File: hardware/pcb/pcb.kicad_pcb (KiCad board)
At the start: 2 copper layers, 20 parts, among them J1 L_GPIO, J2 R_GPIO, J4 USB_C_Receptacle_USB2.0_14P, SW1 SW_Push, SW2 SW_Push, U1 ESP32-C3-WROOM-02, U3 TPS62291

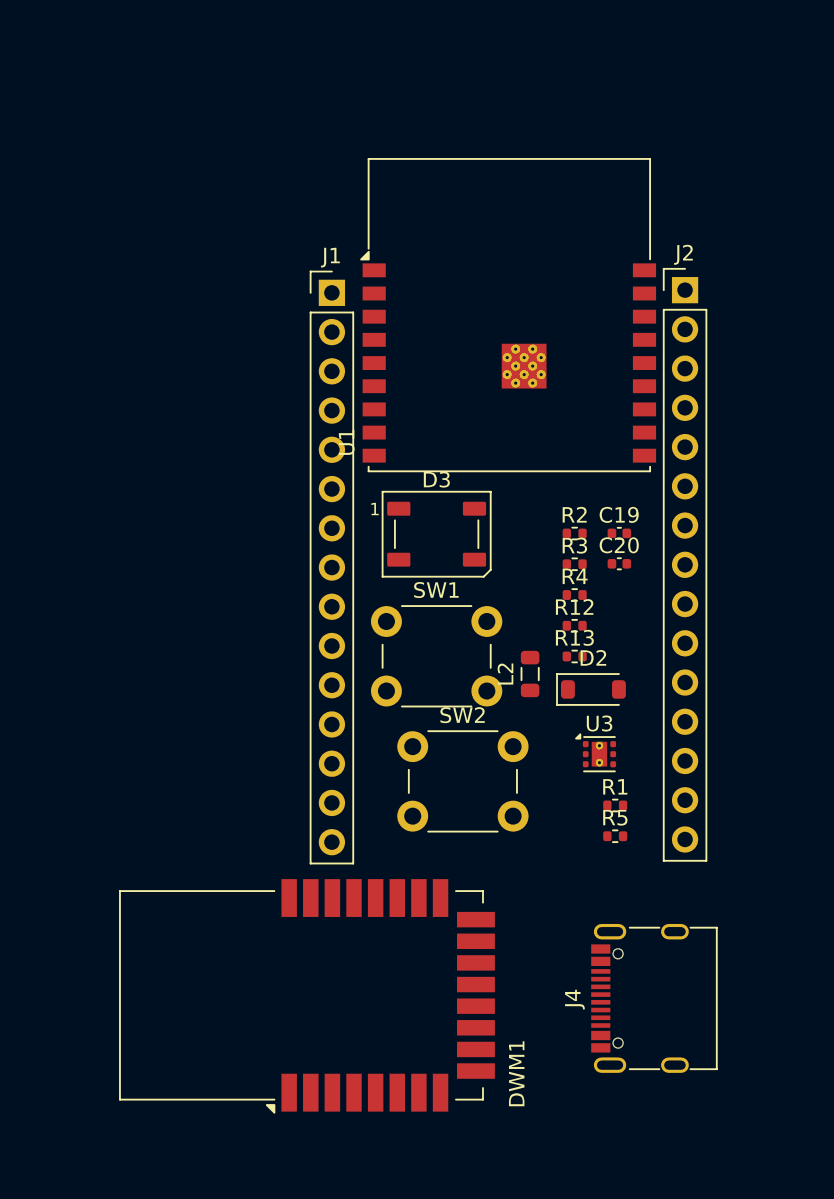
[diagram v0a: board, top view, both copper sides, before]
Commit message: finished schematic and routed pcb
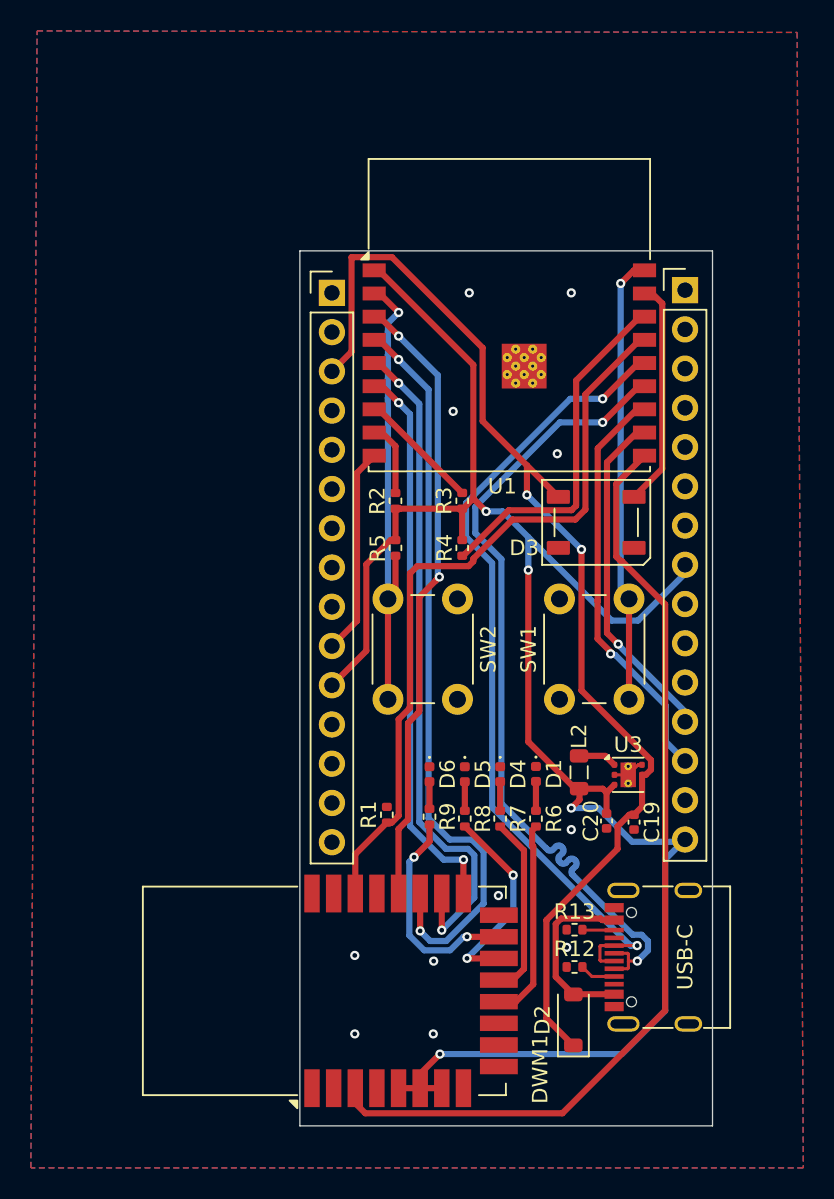
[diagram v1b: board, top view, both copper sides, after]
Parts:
- added D1: TXLED, LED_SMD:LED_0402_1005Metric, F.Cu at (104.6, 83.0)
- added D4: RXLED, LED_SMD:LED_0402_1005Metric, F.Cu at (102.3, 83.0)
- added D5: SFDLED, LED_SMD:LED_0402_1005Metric, F.Cu at (100.0, 83.0)
- added D6: RXOKLED, LED_SMD:LED_0402_1005Metric, F.Cu at (97.8, 83.0)
- added R6: R_Small, Resistor_SMD:R_0402_1005Metric, F.Cu at (104.6, 85.8)
- added R7: R_Small, Resistor_SMD:R_0402_1005Metric, F.Cu at (102.3, 85.8)
- added R8: R_Small, Resistor_SMD:R_0402_1005Metric, F.Cu at (100.0, 85.8)
- added R9: R_Small, Resistor_SMD:R_0402_1005Metric, F.Cu at (97.8, 85.7)
- SW1: value SW_Push -> MODE
- SW2: value SW_Push -> RESET
- moved R5 23.5 mm to (95.6, 68.3), turned to -90 degrees
- moved R12 22.1 mm to (107.1, 95.5)
- moved D2 21.4 mm to (107.1, 98.9), turned to 90 degrees
- moved C19 18.7 mm to (111.0, 86.1), turned to -90 degrees
- moved R13 17.7 mm to (107.1, 93.0)
- moved C20 16.7 mm to (109.2, 86.0), turned to -90 degrees
- moved R1 14.8 mm to (95.0, 85.6), turned to 90 degrees
- moved SW1 12.3 mm to (106.2, 78.1), turned to 90 degrees
- moved R2 11.8 mm to (95.6, 65.3), turned to 90 degrees
- moved D3 10.4 mm to (108.5, 66.7)
- moved SW2 9.99 mm to (99.6, 71.6), turned to -90 degrees
- moved R3 8.36 mm to (99.9, 65.3), turned to 90 degrees
- moved R4 7.89 mm to (99.9, 68.3), turned to 90 degrees
- moved L2 7.11 mm to (107.4, 82.9)
- moved USB-C 2.81 mm to (113.4, 94.8)
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- renumbered J4 to USB-C
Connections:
- DWM1 pad 12: unconnected-(DWM1-GPIO3/TXLED-Pad12) -> /TXLED
- DWM1 pad 13: unconnected-(DWM1-GPIO2/RXLED-Pad13) -> /RXLED
- DWM1 pad 14: unconnected-(DWM1-GPIO1/SFDLED-Pad14) -> /SFDLED
- DWM1 pad 15: unconnected-(DWM1-GPIO0/RXOKLED-Pad15) -> /RXOKLED
- J1 pad 3: VUSB -> +5V
- U1 pad 11: unconnected-(U1-IO20/RXD-Pad11) -> /RXD
- U1 pad 12: unconnected-(U1-IO21/TXD-Pad12) -> /TXD
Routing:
- net +3V3: track 0.00 -> 121.5 mm, vias 0 -> 4
- net +5V: track 0.00 -> 75.2 mm, vias 0 -> 2
- net /U-RSTn: track 0.00 -> 62.1 mm
- net USB_D-: track 0.00 -> 54.4 mm, vias 0 -> 2
- net USB_D+: track 0.00 -> 53.1 mm, vias 0 -> 2
- net /U-IRQ: track 0.00 -> 48.3 mm
- net /U-SPIMISO: track 0.00 -> 48.2 mm, vias 0 -> 2
- net /U-SPIMOSI: track 0.00 -> 43.6 mm, vias 0 -> 2
- net /U-SPICLK: track 0.00 -> 40.4 mm, vias 0 -> 2
- net /U-SPICSn: track 0.00 -> 36.3 mm, vias 0 -> 2
- net /ENABLE: track 0.00 -> 30.4 mm, vias 0 -> 1
- net /BUTTON: track 0.00 -> 29.0 mm, vias 0 -> 1
- net /TXD: track 0.00 -> 26.8 mm, vias 0 -> 1
- net Net-(U1-IO2): track 0.00 -> 23.0 mm
- net /RXD: track 0.00 -> 22.1 mm, vias 0 -> 1
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- added copper zone on B.Cu, net GND
- added copper zone on F.Cu, net GND
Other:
- board outline added: 26.7 x 56.6 mm
